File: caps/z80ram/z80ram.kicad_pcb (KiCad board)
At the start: 4 copper layers, 85 x 56 mm, 19 parts, among them J10 PORTG, J2 PORTA, J3 PORTB, J5 PORTD, J6 PORTE, J7 PORTF, U1 74HCT257, U2 AS6C4008-55PCN, U3 74HCT574, U4 Z80CPU

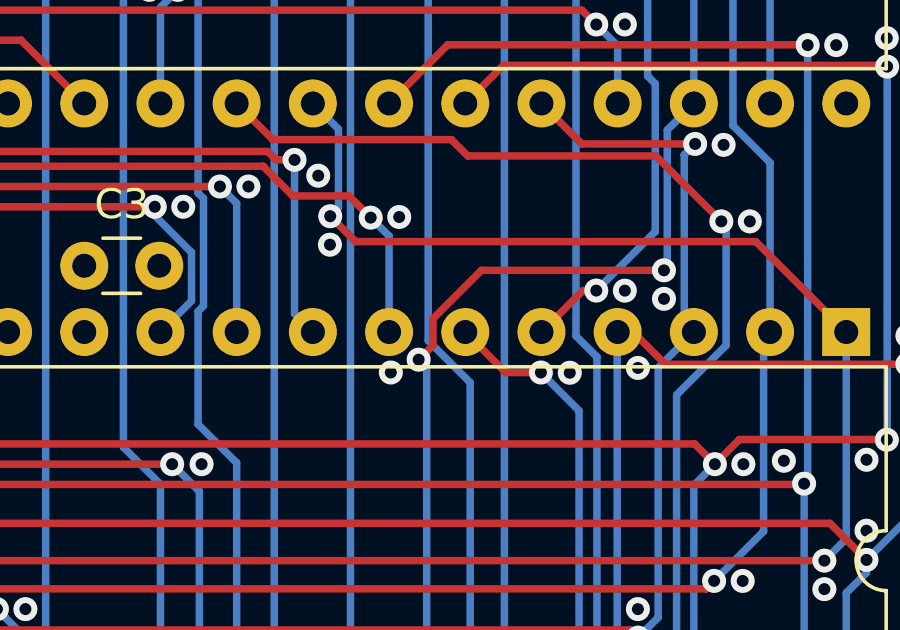
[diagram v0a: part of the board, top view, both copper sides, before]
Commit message: Final (?!) tweaks
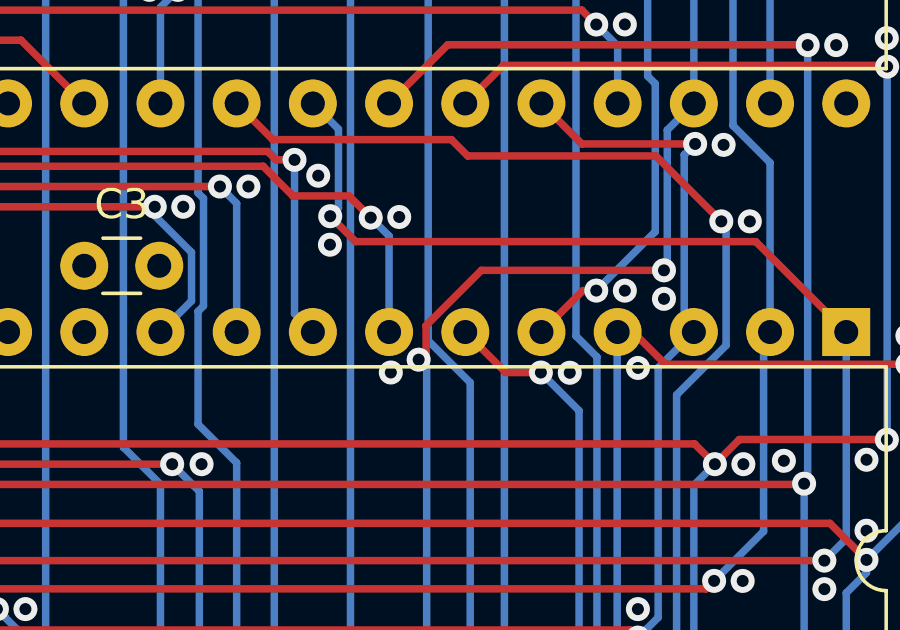
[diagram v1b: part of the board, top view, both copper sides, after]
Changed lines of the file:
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@@
 	)
 	(segment
-		(start 182.481637 110.043082)
-		(end 182.481637 109.15472)
+		(start 182.25 110.274719)
+		(end 182.25 109.386357)
 		(width 0.25)
 		(layer "F.Cu")
@@
 	(segment
 		(start 182.003241 110.521478)
-		(end 182.481637 110.043082)
+		(end 182.25 110.274719)
 		(width 0.25)
 		(layer "F.Cu")
@@
 	)
 	(segment
-		(start 182.481637 109.15472)
+		(start 182.25 109.386357)
 		(end 184.092757 107.5436)
 		(width 0.25)
